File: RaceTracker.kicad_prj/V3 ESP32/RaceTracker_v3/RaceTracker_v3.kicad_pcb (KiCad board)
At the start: 4 copper layers, 50 x 87 mm, 45 parts, among them J1 USB-C, J2 Battery, J3 Qwiic GPS (I2C), J4 microSD, J5 UART Debug, J6 e-Paper (steckbar) 8p, SW1 PWR, SW2 RESET, SW3 BOOT, U1 ESP32-S3-WROOM-1-N8, U2 MCP73831T-2ACI/OT, U3 AP2112K-3.3, U4 WSEN-ISDS

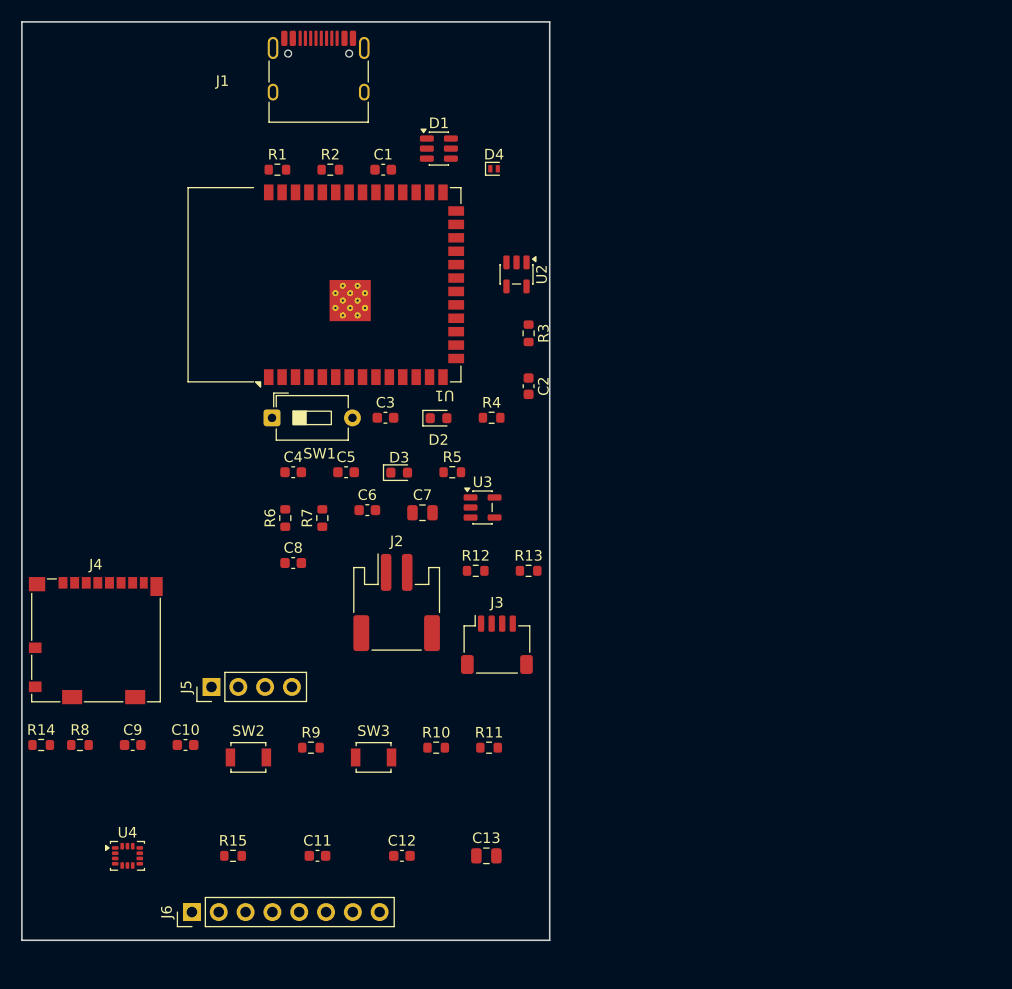
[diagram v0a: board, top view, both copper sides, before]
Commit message: V3: GND/+3V3 Planes, Power-Routing, Teilrouting der Signalnetze
Co-Authored-By: Claude Sonnet 5 <noreply@anthropic.com>
Claude-Session: https://claude.ai/code/session_01KJ1x8W8LsYuDo52VfB14br
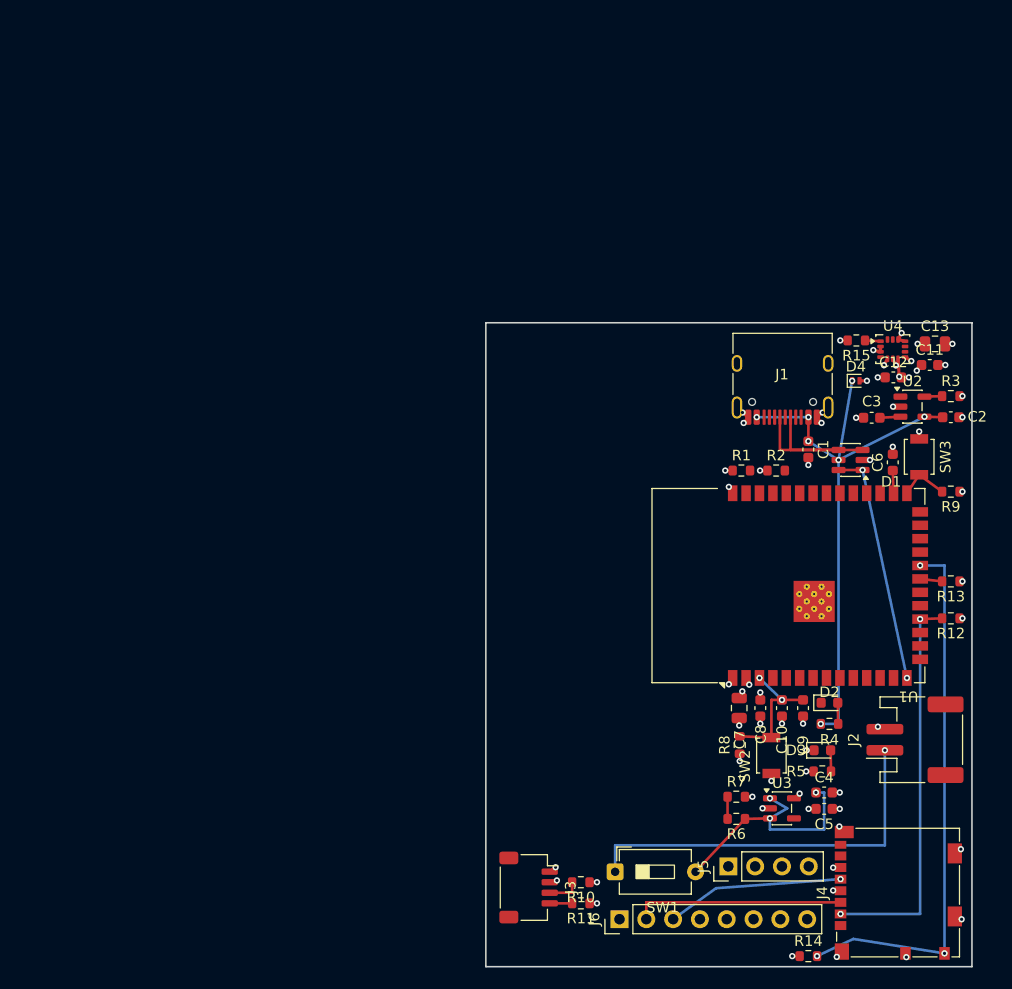
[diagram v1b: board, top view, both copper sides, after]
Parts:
- moved U4 86.9 mm to (82.5, 31.0)
- moved J4 79.7 mm to (83.0, 82.5), turned to 90 degrees
- moved R15 76.6 mm to (79.0, 30.2), turned to 180 degrees
- moved R14 75.4 mm to (74.5, 88.5)
- moved C11 74.3 mm to (86.0, 32.5)
- moved R9 65.3 mm to (88.0, 44.5), turned to 180 degrees
- moved C12 65.0 mm to (82.5, 33.7)
- moved C13 64.5 mm to (86.5, 30.5)
- moved C9 63.6 mm to (74.0, 65.0), turned to 90 degrees
- moved R8 62.5 mm to (68.0, 68.5), turned to 90 degrees
- moved SW3 59.0 mm to (85.0, 41.2), turned to -90 degrees
- moved C4 58.7 mm to (76.0, 73.0)
- moved C10 56.6 mm to (72.0, 65.0), turned to 90 degrees
- moved C5 55.4 mm to (76.0, 74.5)
- moved SW1 53.9 mm to (56.2, 80.5)
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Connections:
- R1 pad 1: Net-(J1-CC1) -> /GND
- R1 pad 2: /GND -> Net-(J1-CC1)
- R2 pad 1: Net-(J1-CC2) -> /GND
- R2 pad 2: /GND -> Net-(J1-CC2)
- U1 pad 4: (no net) -> /EPD_CS
- U1 pad 5: (no net) -> /EPD_DC
- U1 pad 6: (no net) -> /EPD_RST
- U1 pad 7: (no net) -> /EPD_BUSY
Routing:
- net /+VBUS: track 0.00 -> 55.7 mm, vias 0 -> 7
- net /SD_CD: track 0.00 -> 51.6 mm, vias 0 -> 3
- net /+VBAT_RAW: track 0.00 -> 39.0 mm, vias 0 -> 1
- net /SD_CS: track 0.00 -> 37.6 mm, vias 0 -> 2
- net /GND: track 0.00 -> 28.6 mm, vias 0 -> 41
- net /+VBAT_SYS: track 0.00 -> 23.5 mm, vias 0 -> 3
- net /USB_DP: track 0.00 -> 22.4 mm, vias 0 -> 2
- net /SD_MOSI: track 0.00 -> 20.0 mm
- net /USB_DM: track 0.00 -> 18.6 mm
- net /SD_SCK: track 0.00 -> 16.8 mm, vias 0 -> 1
- net /+3V3: track 0.00 -> 15.3 mm, vias 0 -> 22
- net Net-(U1-EN): track 0.00 -> 12.6 mm, vias 0 -> 2
- net Net-(U1-IO0): track 0.00 -> 4.80 mm
- net /BATT_SENSE: track 0.00 -> 4.25 mm
- net /I2C_SDA: track 0.00 -> 3.12 mm
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- added copper zone on In2.Cu, net /+3V3
- added copper zone on In1.Cu, net /GND
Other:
- board size 50 x 87 mm -> 46 x 61 mm
